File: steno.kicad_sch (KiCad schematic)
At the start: 13 parts, among them J2 USB_C_Receptacle_USB2.0_16P, U1 W25Q16JVSS, U2 AMS1117-3.3

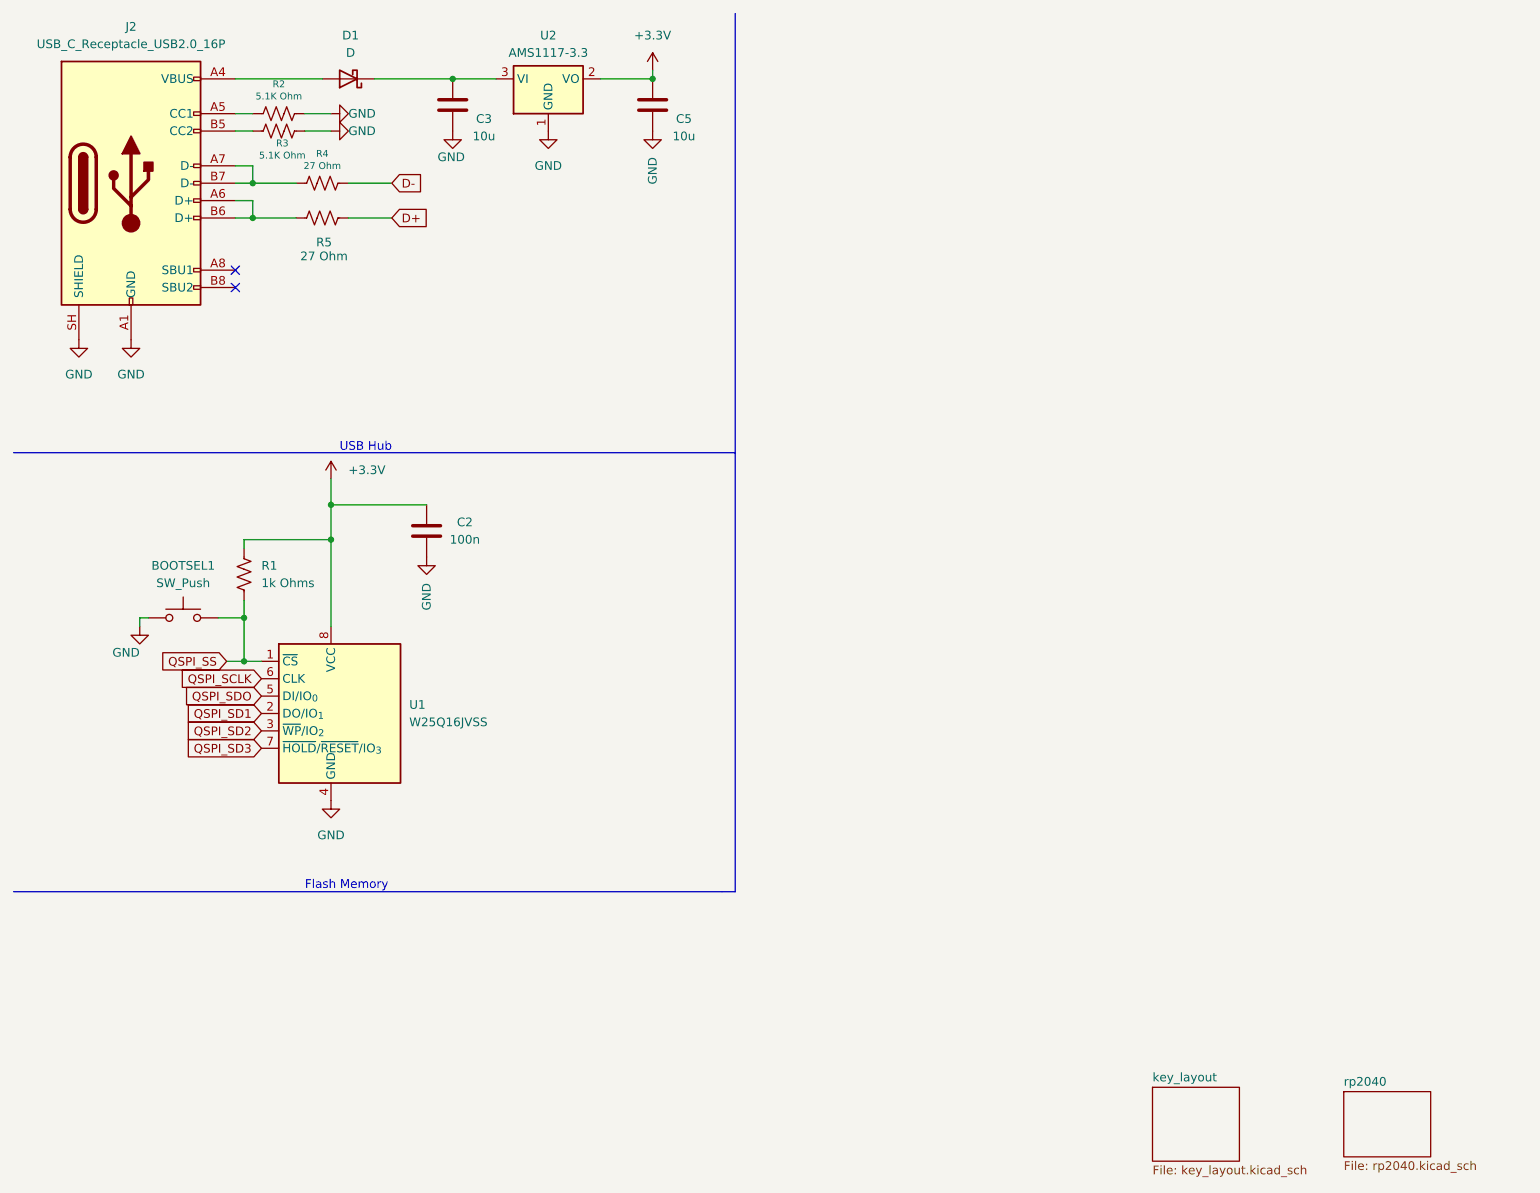
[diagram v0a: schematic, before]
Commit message: Init Commit!
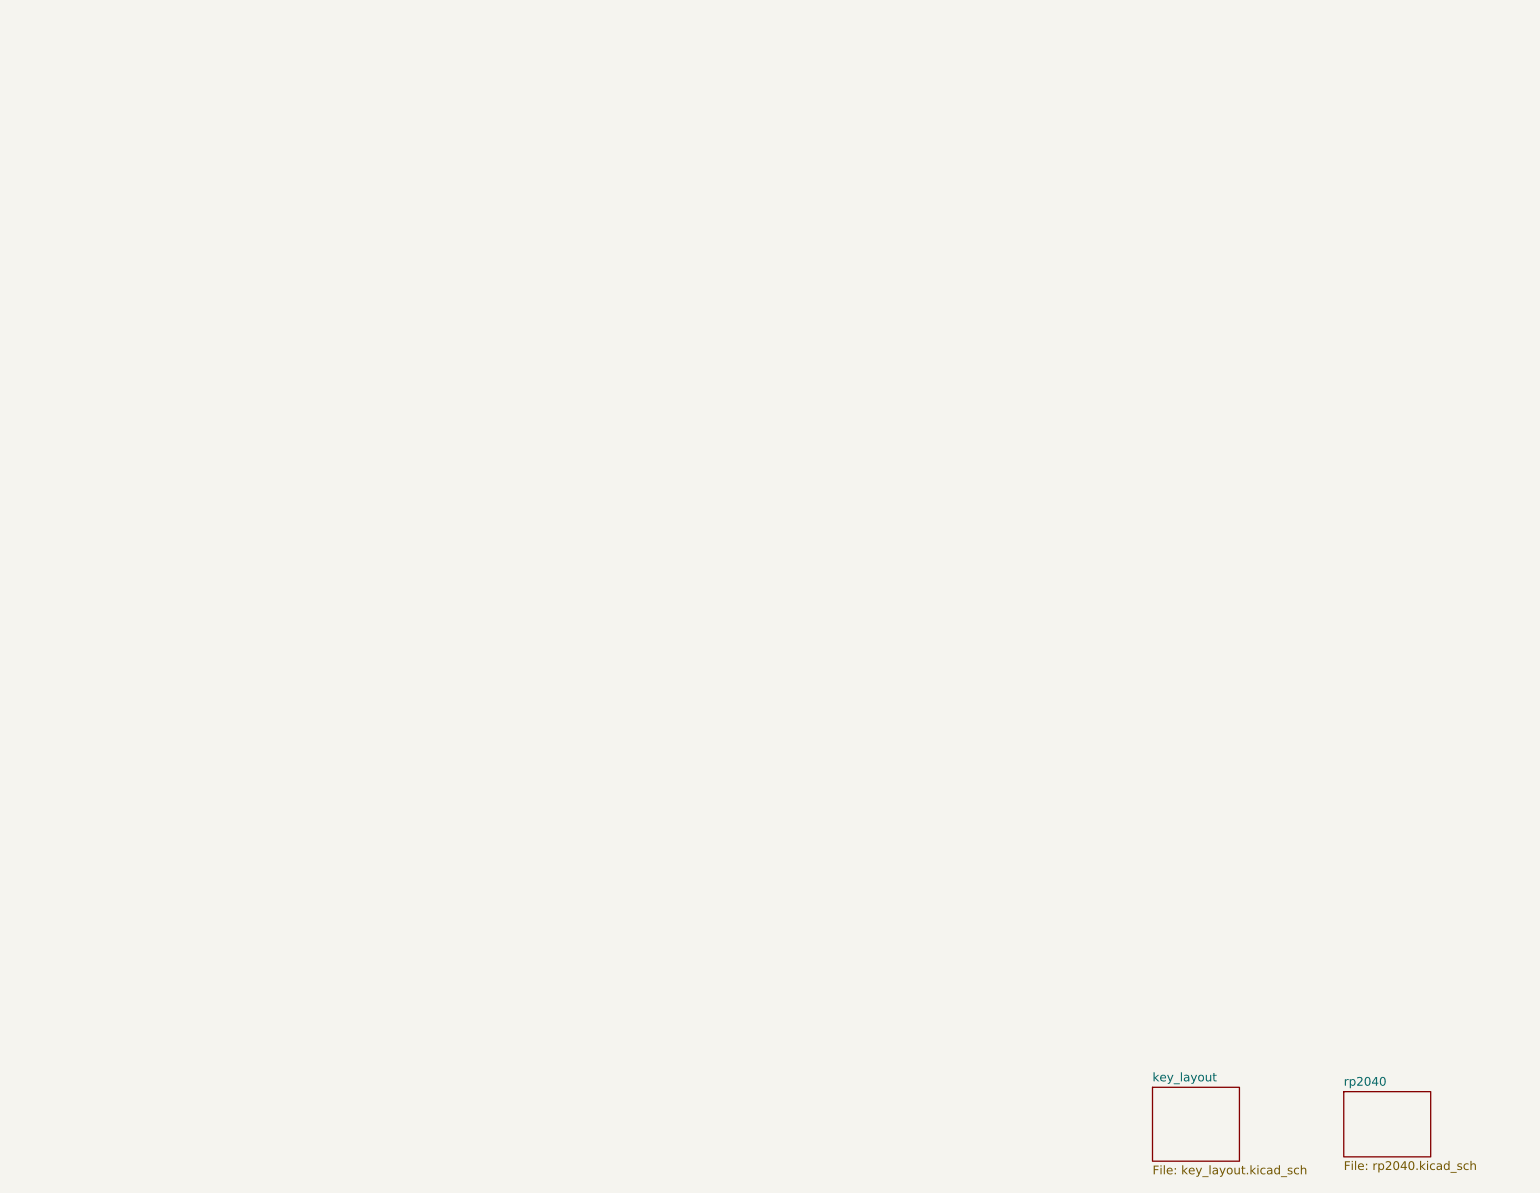
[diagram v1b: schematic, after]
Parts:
- removed BOOTSEL1: SW_Push, 3rd_party_footprints:SW4_PTS815 SJM 250 SMTR LFS_CNK, symbol Switch:SW_Push
- removed C2: 100n, Capacitor_SMD:C_0402_1005Metric, symbol Device:C
- removed C3, C5: 10u, Capacitor_SMD:C_0603_1608Metric, symbol Device:C
- removed D1: D, Diode_SMD:D_SMA, symbol Device:D_Schottky
- removed J2: USB_C_Receptacle_USB2.0_16P, Connector_USB:USB_C_Receptacle_HCTL_HC-TYPE-C-16P-01A, symbol Connector:USB_C_Receptacle_USB2.0_16P
- removed R1: 1k Ohms, Resistor_SMD:R_0402_1005Metric, symbol Device:R_US
- removed R2, R3: 5.1K Ohm, Resistor_SMD:R_0402_1005Metric, symbol Device:R_US
- removed R4, R5: 27 Ohm, Resistor_SMD:R_0402_1005Metric, symbol Device:R_US
- removed U1: W25Q16JVSS, Package_SO:SOIC-8_5.3x5.3mm_P1.27mm, symbol Memory_Flash:W25Q16JVSS
- removed U2: AMS1117-3.3, Package_TO_SOT_SMD:SOT-223-3_TabPin2, symbol Regulator_Linear:AMS1117-3.3
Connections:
- no-connect marks 2 -> 0
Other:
- note removed: "Flash Memory"
- note removed: "USB Hub"
